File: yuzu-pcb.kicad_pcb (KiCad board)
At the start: 2 copper layers, 25 x 27 mm, 14 parts, among them J1 Conn_ARM_JTAG_SWD_10, M1 MountingHole_2.5mm, M2 MountingHole_2.5mm, SW1 SW_SPST, U1 E73-2G4M08S1C, U2 SHT45, X2 32.768Khz

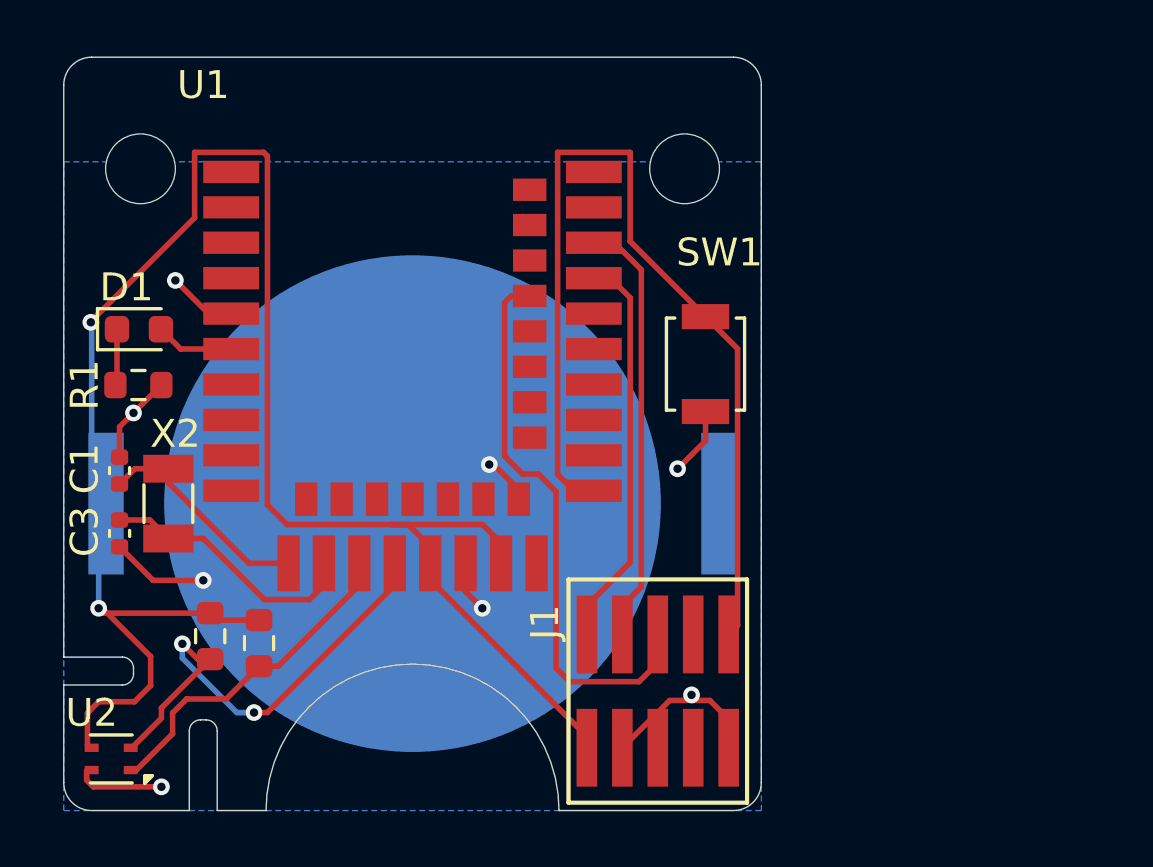
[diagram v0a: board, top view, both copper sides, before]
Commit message: Updated schematic and pcb
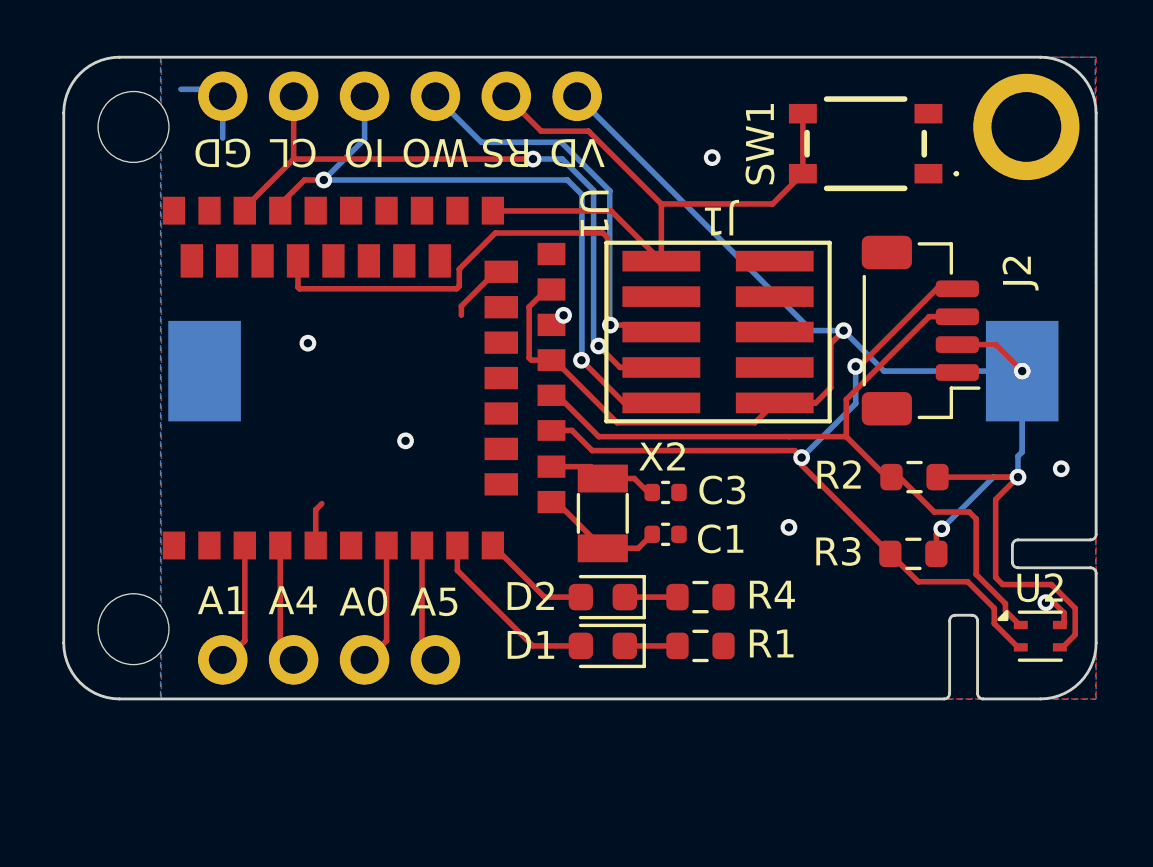
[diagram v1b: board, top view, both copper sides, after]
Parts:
- removed M1, M2: MountingHole_2.5mm, MountingHole:MountingHole_2.5mm
- added D2: White, LED_SMD:LED_0603_1608Metric, F.Cu at (119.3, 119.3)
- added J2: Conn_01x04, Connector_JST:JST_SH_BM04B-SRSS-TB_1x04-1MP_P1.00mm_Vertical, F.Cu at (130.7, 109.8)
- added R4: 1K, Resistor_SMD:R_0603_1608Metric, F.Cu at (122.8, 119.3)
- added REF**: MountingHole_2.5mm, yuzu:MountingHole_2.5mm, F.Cu at (102.5, 120.5)
- added REF**: MountingHole_2.5mm_Pad, yuzu:MountingHole_2.5mm_Pad, F.Cu at (134.5, 102.5)
- added REF**: MountingHole_2.5mm, yuzu:MountingHole_2.5mm, F.Cu at (102.5, 102.5)
- added TP1: A1, yuzu:TestPoint_THTPad, F.Cu at (105.7, 121.6)
- added TP10: VD, yuzu:TestPoint_THTPad, F.Cu at (118.4, 101.4)
- added TP2: A4, yuzu:TestPoint_THTPad, F.Cu at (108.2, 121.6)
- added TP3: A0, yuzu:TestPoint_THTPad, F.Cu at (110.8, 121.6)
- added TP4: A5, yuzu:TestPoint_THTPad, F.Cu at (113.3, 121.6)
- added TP5: GD, yuzu:TestPoint_THTPad, F.Cu at (105.7, 101.4)
- added TP6: CL, yuzu:TestPoint_THTPad, F.Cu at (108.2, 101.4)
- added TP7: IO, yuzu:TestPoint_THTPad, F.Cu at (110.8, 101.4)
- added TP8: WO, yuzu:TestPoint_THTPad, F.Cu at (113.3, 101.4)
- added TP9: RS, yuzu:TestPoint_THTPad, F.Cu at (115.9, 101.4)
- BT1: footprint Battery:BatteryHolder_Keystone_3034_1x20mm -> Battery:BatteryHolder_Keystone_1060_1x2032
- SW1: footprint Button_Switch_SMD:SW_SPST_B3U-1000P -> yuzu:RKB2SJG250SMTRLFS
- U1: footprint yuzu:E73(2G4M08S1C) JLCPCB -> yuzu:E73(2G4M08S1C) JLCPCB_2
- moved U2 33.6 mm to (135.0, 120.8), turned to 0 degrees
- moved R3 25.4 mm to (130.4, 117.8), turned to 180 degrees
- moved R2 24.2 mm to (130.5, 115.0), turned to 180 degrees
- moved R1 22.2 mm to (122.8, 121.1)
- moved D1 20.1 mm to (119.3, 121.1), turned to 180 degrees
- moved C1 19.7 mm to (121.6, 117.1), turned to 0 degrees
- moved C3 19.6 mm to (121.6, 115.6), turned to 0 degrees
- moved X2 15.6 mm to (119.3, 116.3), turned to 90 degrees
- moved J1 13.0 mm to (123.5, 109.8), turned to 90 degrees
- moved SW1 9.77 mm to (128.7, 103.1), turned to 180 degrees
- moved BT1 8.63 mm to (119.7, 111.2)
- moved U1 4.24 mm to (109.0, 111.5), turned to -90 degrees
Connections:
- net Net-(U1-P0.00/XL1) renamed /XL1
- net Net-(U1-P0.01/XL2) renamed /XL2
- U1 pad 10: unconnected-(U1-P0.30/AIN6-Pad10) -> /WHITE_LED
- U1 pad 15: /SDA -> /SCL
- U1 pad 17: /SCL -> /SDA
- U1 pad 3: unconnected-(U1-P0.03/AIN1-Pad3) -> Net-(U1-P0.03/AIN1)
- U1 pad 4: unconnected-(U1-P0.28/AIN4-Pad4) -> Net-(U1-P0.28/AIN4)
- U1 pad 6: /RED_LED -> unconnected-(U1-P1.13-Pad6)
- U1 pad 7: unconnected-(U1-P0.02/AIN0-Pad7) -> Net-(U1-P0.02/AIN0)
- U1 pad 8: unconnected-(U1-P0.29/AIN5-Pad8) -> Net-(U1-P0.29/AIN5)
- U1 pad 9: unconnected-(U1-P0.31/AIN7-Pad9) -> /RED_LED
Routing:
- net /SDA: track 12.2 -> 28.1 mm
- net GND: track 24.6 -> 8.86 mm, vias 8 -> 7
- net /SCL: track 17.2 -> 29.4 mm
- net /RESET: track 34.7 -> 23.7 mm
- net /SWO: track 20.3 -> 30.9 mm, vias 0 -> 1
- net /SWDIO: track 14.3 -> 24.7 mm, vias 0 -> 2
- net /SWCLK: track 15.4 -> 24.3 mm, vias 0 -> 2
- net /nrf_VDD: track 67.9 -> 60.3 mm, vias 2 -> 4
- net /XL2: track 9.52 -> 3.99 mm
- net Net-(U1-P0.03/AIN1): track 0.00 -> 4.53 mm
- net Net-(U1-P0.02/AIN0): track 0.00 -> 4.53 mm
- net Net-(U1-P0.29/AIN5): track 0.00 -> 4.40 mm
- net Net-(U1-P0.28/AIN4): track 0.00 -> 4.40 mm
- net /WHITE_LED: track 0.00 -> 3.92 mm
- net /RED_LED: track 2.86 -> 6.44 mm
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- added copper zone on F.Cu, net GND
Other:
- board size 25 x 27 mm -> 37 x 23 mm
- board text added: "YUZU [${REV}]"
